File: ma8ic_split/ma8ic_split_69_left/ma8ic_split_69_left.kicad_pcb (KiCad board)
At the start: 2 copper layers, 166.3 x 125.7 mm, 133 parts, among them J1 USB_C_Receptacle, J2 MJ-4PP-9, J3 I2C, J4 SPI, SW1 SW_PUSH, SW10 SW_PUSH-kbd, SW11 SW_PUSH-kbd, SW12 SW_PUSH-kbd, SW13 SW_PUSH-kbd, SW14 SW_PUSH-kbd, SW15 SW_PUSH-kbd, SW16 SW_PUSH-kbd, SW17 SW_PUSH-kbd, SW18 SW_PUSH-kbd, SW19 SW_PUSH-kbd, SW2 SW_PUSH-kbd, SW20 SW_PUSH-kbd, SW21 SW_PUSH-kbd, SW22 SW_PUSH-kbd, SW23 SW_PUSH-kbd, SW24 SW_PUSH-kbd, SW25 SW_PUSH-kbd, SW26 SW_PUSH-kbd, SW27 SW_PUSH-kbd, SW28 SW_PUSH-kbd, SW29 SW_PUSH-kbd, SW3 SW_PUSH-kbd, SW30 SW_PUSH-kbd, SW31 SW_PUSH-kbd, SW32 SW_PUSH-kbd, SW33 SW_PUSH-kbd, SW4 SW_PUSH-kbd, SW5 SW_PUSH-kbd, SW6 SW_PUSH-kbd, SW7 SW_PUSH-kbd, SW8 SW_PUSH-kbd, SW9 SW_PUSH-kbd, U1 ATMEGA32U4, X1 CSTNE16M0V530000R0

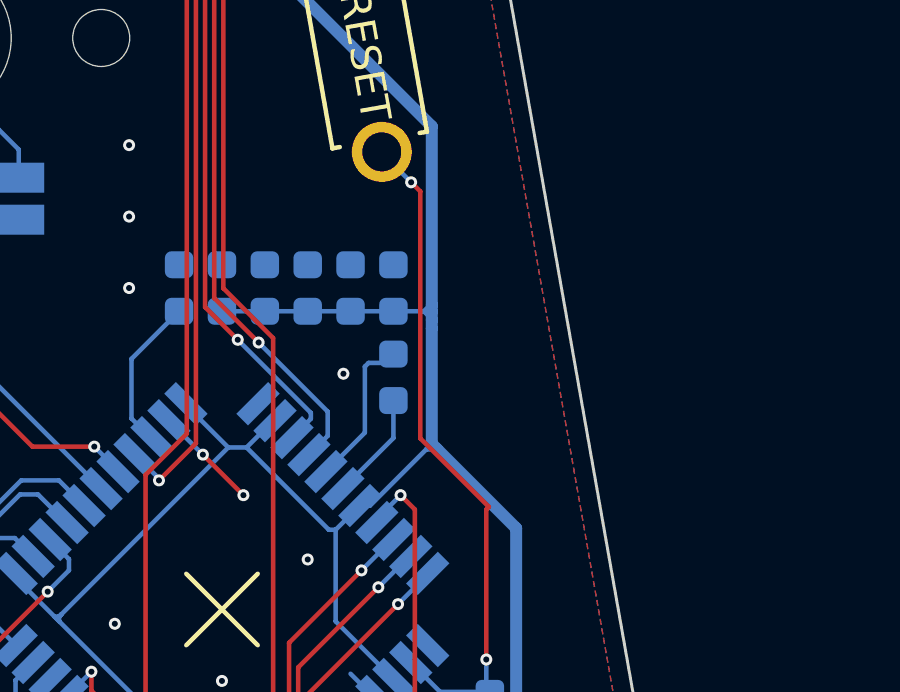
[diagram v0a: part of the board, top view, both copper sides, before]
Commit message: update
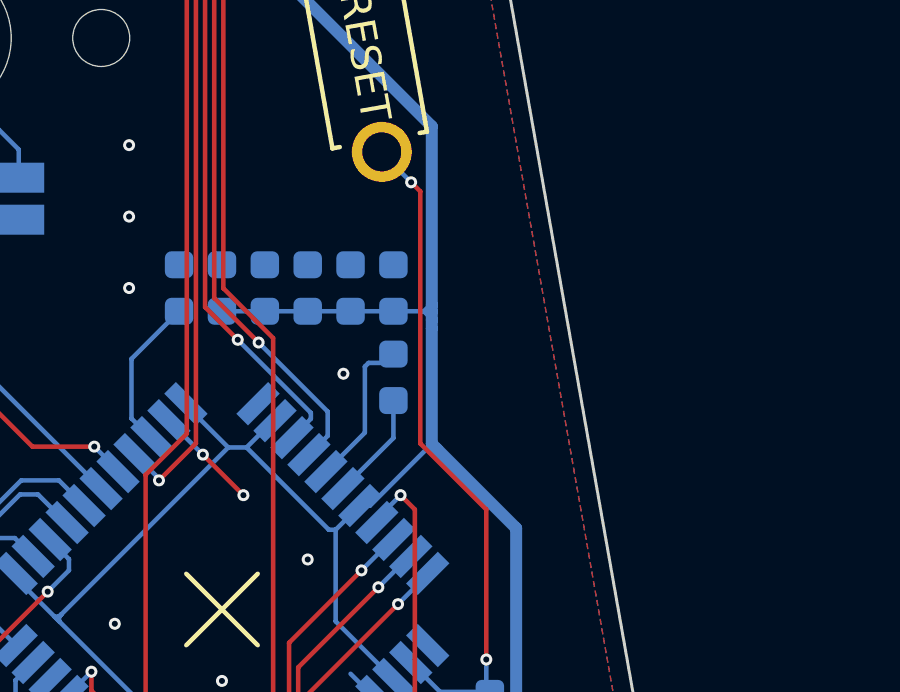
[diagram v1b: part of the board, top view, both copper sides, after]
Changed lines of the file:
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@@
     (pts (xy 183.594375 29.765625) (xy 183.574497 155.438553))
     (height -44.786972)
-    (gr_text "125.6729 mm" (at 227.221407 92.608991 89.99093738) (layer "Dwgs.User")
+    (gr_text "4.9478 in" (at 227.221407 92.608991 89.99093738) (layer "Dwgs.User")
       (effects (font (size 1 1) (thickness 0.15)))
     )
@@
     (pts (xy 214.074375 124.539375) (xy 47.625 124.539375))
     (height 102.631875)
-    (gr_text "166.4494 mm" (at 130.849688 20.7575) (layer "Dwgs.User")
+    (gr_text "6.5531 in" (at 130.849688 20.7575) (layer "Dwgs.User")
       (effects (font (size 1 1) (thickness 0.15)))
     )
@@
   (segment (start 198.043392 76.872884) (end 198.043392 76.752858) (width 0.1524) (layer "B.Cu") (net 99))
   (segment (start 200.50125 95.25) (end 201.224064 95.25) (width 0.1524) (layer "B.Cu") (net 99))
-  (segment (start 199.4916 65.8368) (end 199.1868 65.532) (width 0.1524) (layer "F.Cu") (net 100))
-  (segment (start 201.7776 76.3524) (end 199.4916 74.0664) (width 0.1524) (layer "F.Cu") (net 100))
+  (segment (start 199.1868 65.532) (end 199.4916 65.8368) (width 0.1524) (layer "F.Cu") (net 100))
   (segment (start 201.691875 76.438125) (end 201.691875 81.43875) (width 0.1524) (layer "F.Cu") (net 100))
-  (segment (start 199.4916 74.0664) (end 199.4916 65.8368) (width 0.1524) (layer "F.Cu") (net 100))
-  (segment (start 201.7776 76.3524) (end 201.691875 76.438125) (width 0.1524) (layer "F.Cu") (net 100))
+  (segment (start 199.4916 74.23785) (end 201.691875 76.438125) (width 0.1524) (layer "F.Cu") (net 100))
+  (segment (start 199.4916 65.8368) (end 199.4916 74.23785) (width 0.1524) (layer "F.Cu") (net 100))
   (via (at 201.691875 81.43875) (size 0.4) (drill 0.2) (layers "F.Cu" "B.Cu") (net 100))
   (via (at 199.1868 65.532) (size 0.4) (drill 0.2) (layers "F.Cu" "B.Cu") (net 100))

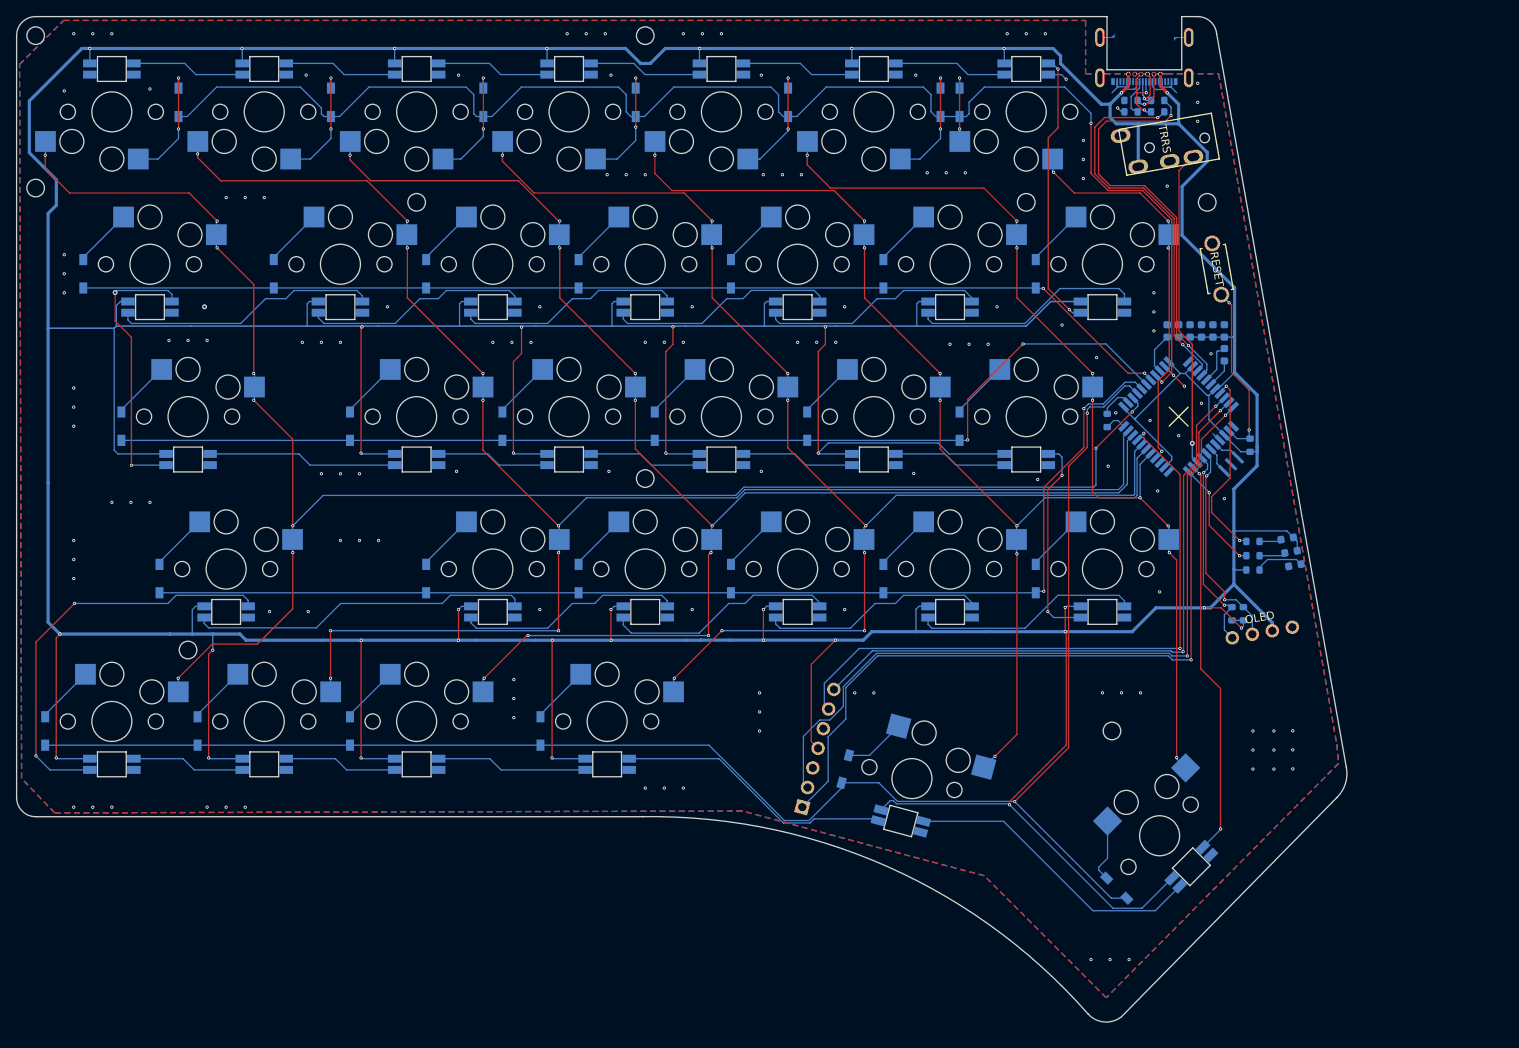
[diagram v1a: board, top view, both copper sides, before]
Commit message: update
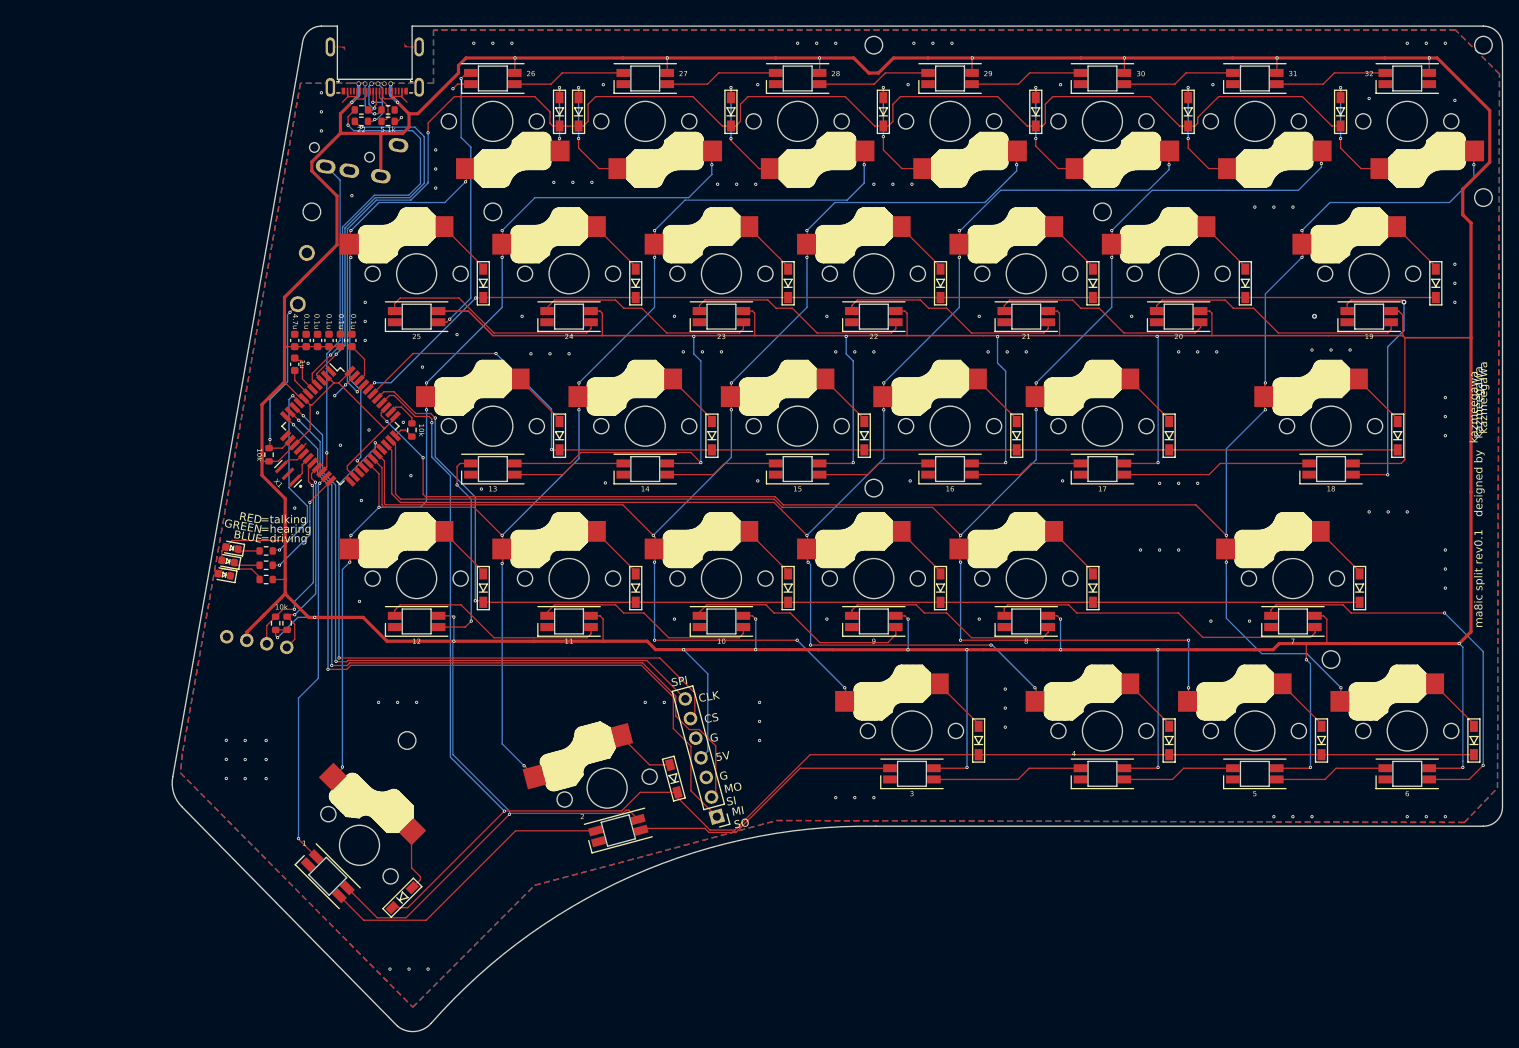
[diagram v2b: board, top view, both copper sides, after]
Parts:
- ? (x5), J2, J3, REF** (x4), SW1, SW10, SW11, SW12, SW13, SW14, SW15, SW16, SW17, SW18, SW19, SW2, SW20, SW21, SW22, SW23, SW24, SW25, SW26, SW27, SW28, SW29, SW3, SW30, SW31, SW32, SW33, SW4, SW5, SW6, SW7, SW8, SW9: moved to B.Cu
- C1, C2, C3, C4, C5, C6, C7, D1, D10, D11, D12, D13, D14, D15, D16, D17, D18, D19, D2, D20, D21, D22, D23, D24, D25, D26, D27, D28, D29, D3, D30, D31, D32, D33, D34, D35, D36, D37, D38, D39, D4, D40, D41, D42, D43, D44, D45, D46, D47, D48, D49, D5, D50, D51, D52, D53, D54, D55, D56, D57, D58, D59, D6, D60, D61, D62, D63, D64, D65, D66, D67, D7, D8, D9, J1, J4, R1, R10, R11, R2, R3, R4, R5, R6, R7, R8, R9, U1, X1: moved to F.Cu
- moved ? 181.0 mm to (231.0, 33.3), turned to 180 degrees
- moved ? 181.0 mm to (231.0, 52.4), turned to 180 degrees
- moved D30 178.6 mm to (229.8, 120.3)
- moved D11 169.1 mm to (225.0, 63.1)
- moved SW2 161.9 mm to (221.5, 42.9), turned to 180 degrees
- moved SW28 161.9 mm to (221.5, 119.1), turned to 0 degrees
- moved D41 161.9 mm to (221.5, 124.4), turned to 0 degrees
- moved D67 161.9 mm to (221.5, 37.5), turned to 0 degrees
- moved D18 159.5 mm to (220.3, 82.2)
- moved SW9 152.4 mm to (216.7, 61.9), turned to 0 degrees
- moved D54 152.4 mm to (216.7, 67.3), turned to 0 degrees
- moved D24 150.0 mm to (215.5, 101.2)
- moved D4 145.3 mm to (213.1, 41.7)
- moved SW16 142.9 mm to (211.9, 81.0), turned to 0 degrees
- moved REF** 142.9 mm to (211.9, 110.1), turned to 180 degrees
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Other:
- outline, holes or cut-outs redrawn
